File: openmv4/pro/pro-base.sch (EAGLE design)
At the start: 172 parts, among them J2 SAMTEC_FTSH-105-01-F-DVSAMTEC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, J7 MURATA_MM8130-2600RA2MURATA_M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, M1 9774030243R, M2 9774030243R, Q1 BSS138, Q2 AO3401, U1 W25Q256JVEIQ_TR, U10 STM32H743IIK6, U11 TEXAS_INSTRUMENTS_BQ24072TRGT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, U12 MICROCHIP_ATECC608A-SSHDA-BMI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, U14 IS42S32800, U2 EMIF06-MSD02N16, U3 ME6211C18M5G, U4 PAM2305AABADJ, U5 LSM6DS3TR-C, U6 MICROCHIP_USB3320C-EZK-TRMICR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, U7 LBEE5KL1DX-TEMP, U8 STMICROELECTRONICS_VL53L1CXV0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, U9 NXP_SEMICONDUCTORS_SE050C2HQ1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, X2 USD-1040310811, X3 DF12-36-DS, X4 S2B-PH-K-S(LF)(SN), Y0 SITIME_SIT1533AI-H4-DCC-32.76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, Y1 DSC1001BI1-024.0000

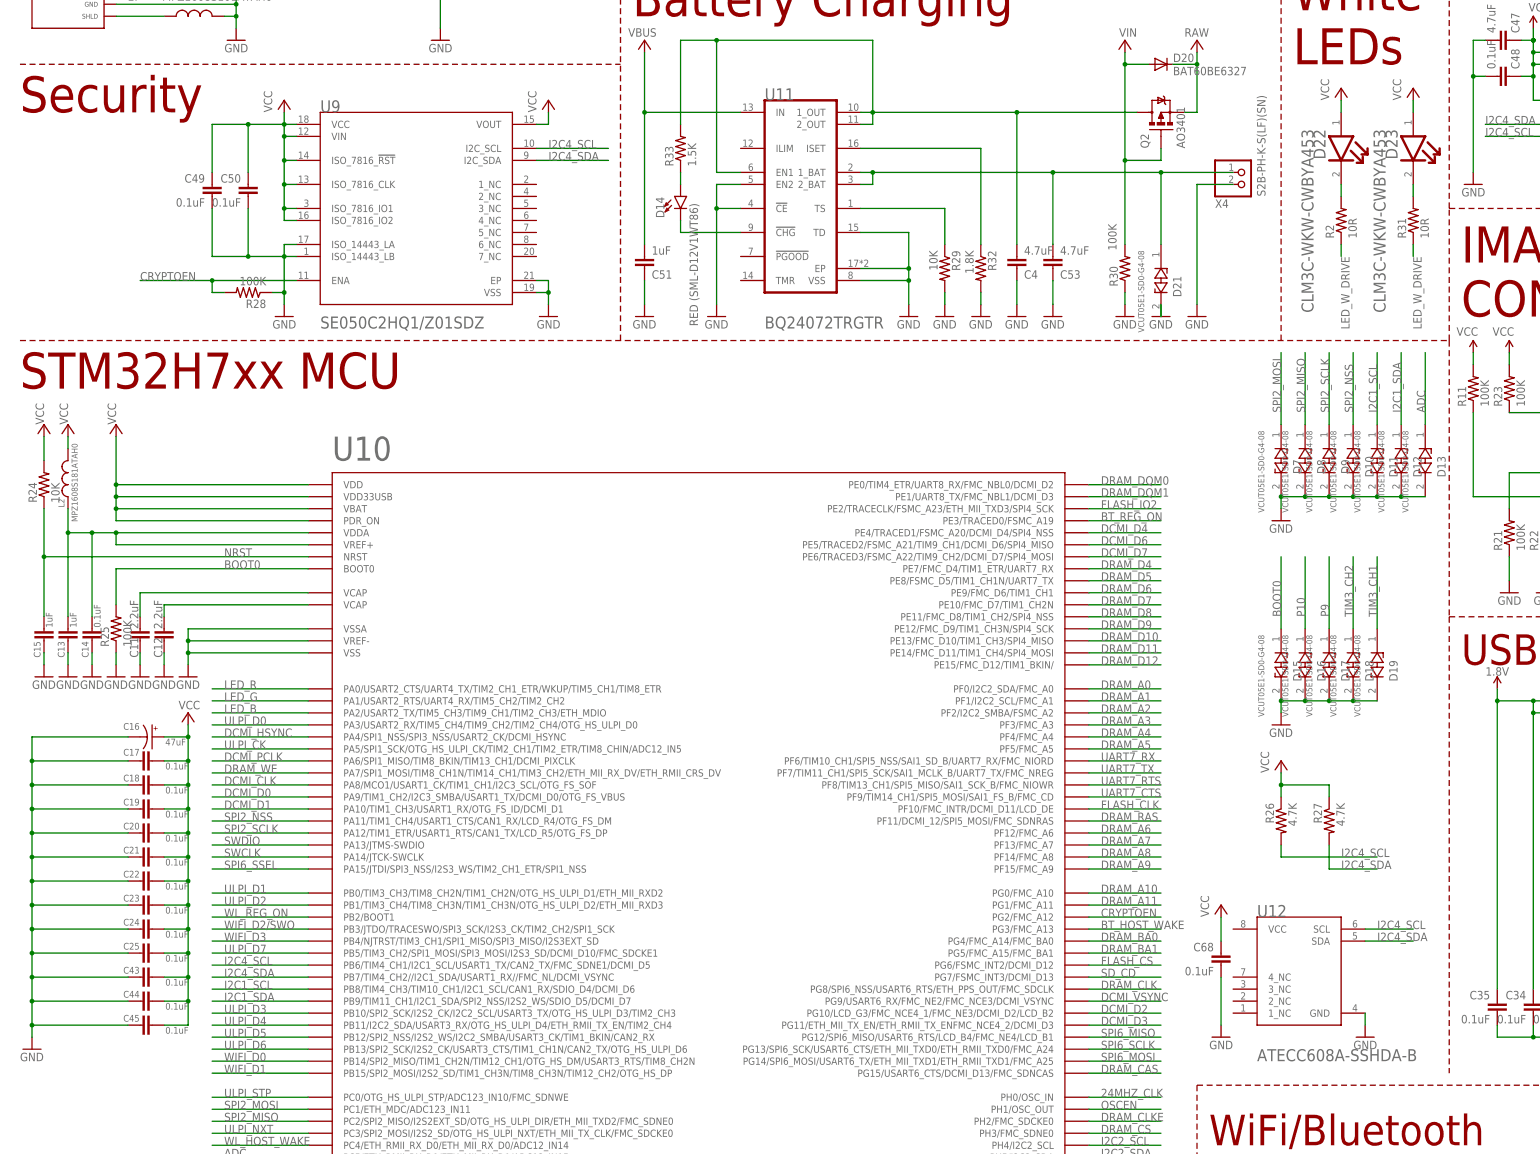
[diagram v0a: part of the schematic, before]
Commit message: Remove NXP chip
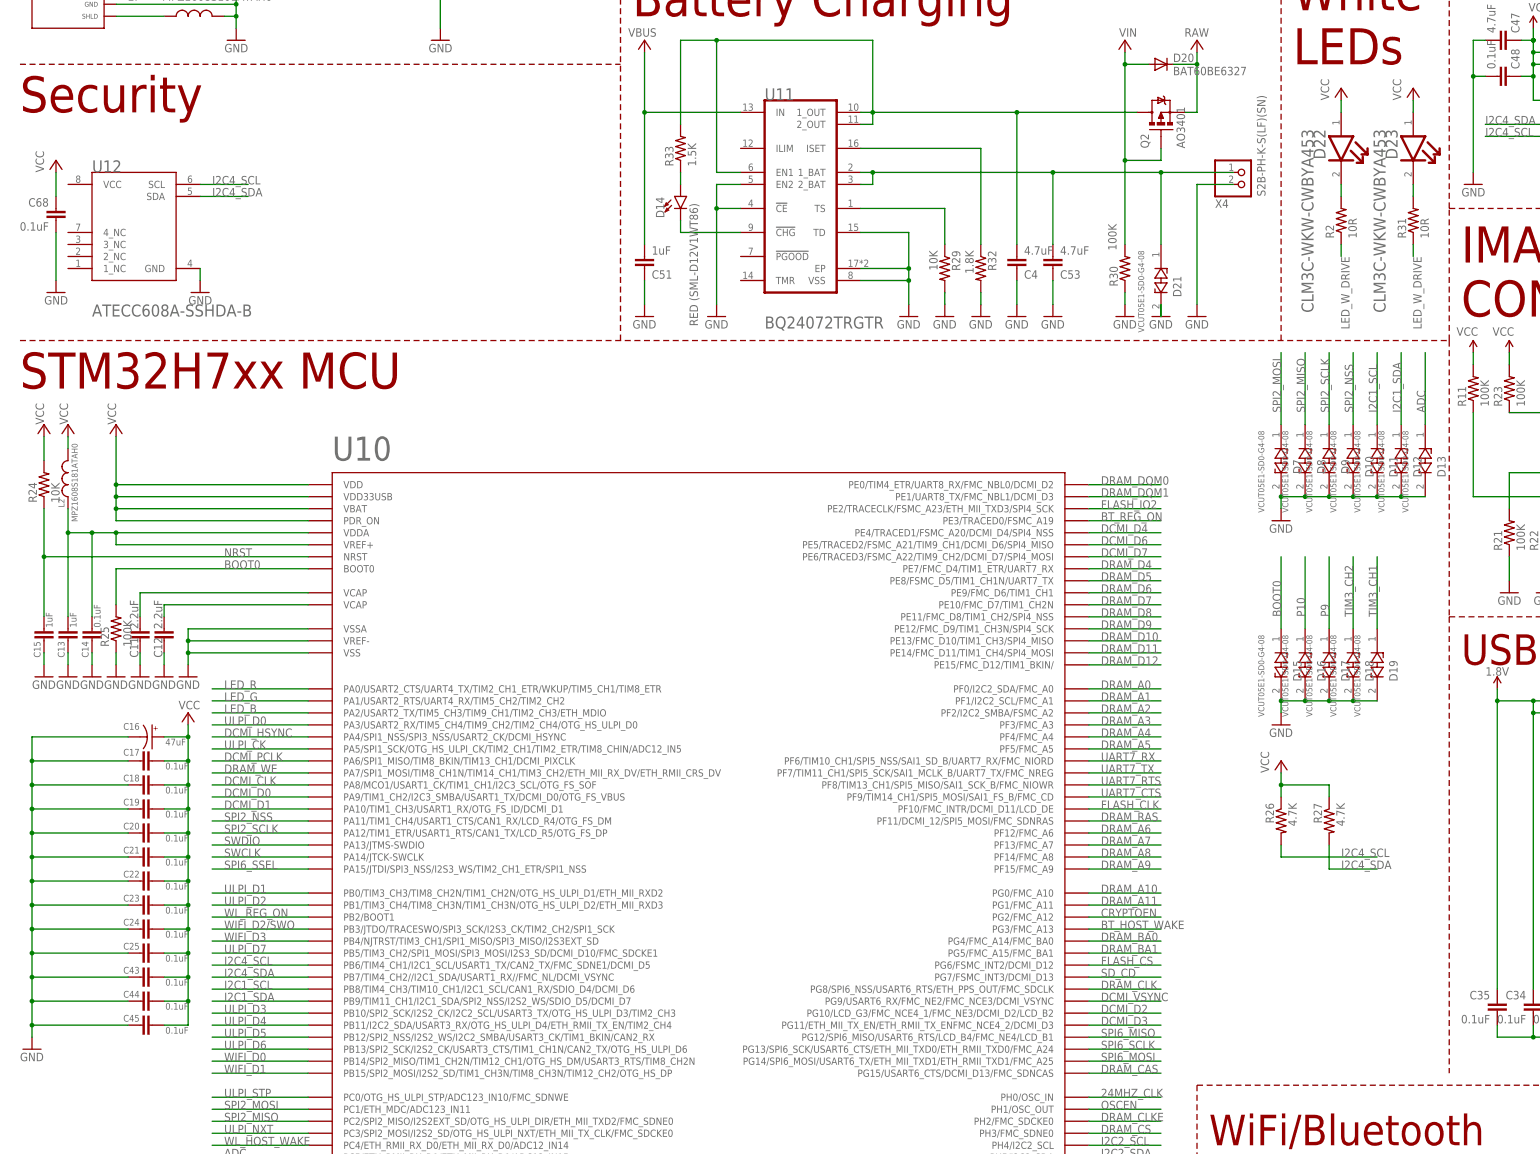
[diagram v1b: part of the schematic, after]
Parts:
- removed C49, C50: 0.1uF, sfe:CAP0402-CAP
- removed R28: 100K, sfe:RESISTOR0402-RES
- removed U9: NXP_SEMICONDUCTORS_SE050C2HQ1-Z01SDZNXP_SEMICONDUCTORS_SE05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, Z01SDZ:NXP_SEMICONDUCTORS_SE050C2HQ1-Z01SDZNXP_SEMICONDUCTORS_SE050C2HQ1-Z01SDZ_0_1
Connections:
- net CRYPTOEN: no longer R28.2, U9.ENA
- net GND: no longer C49.2, C50.2, R28.1, U9.EP, U9.ISO_14443_LA, U9.ISO_14443_LB, U9.VSS
- net I2C4_SCL: no longer U9.I2C_SCL
- net I2C4_SDA: no longer U9.I2C_SDA
- net VCC: no longer C49.1, C50.1, U9.ISO_7816_!RST!, U9.ISO_7816_CLK, U9.ISO_7816_IO1, U9.ISO_7816_IO2, U9.VCC, U9.VIN, U9.VOUT
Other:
- moved on the sheet: C68, U12
